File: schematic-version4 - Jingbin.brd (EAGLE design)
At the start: 47 x 28 mm, 54 parts, among them J2 FTDI_DEVICE, M1 WIRELESS-NRF24L01, Q1 8MHz, T1 NMOS, T2 NMOS, T3 NMOS, T4 NMOS, U1 ATMEGA328P_TQFP, U2 GY-521MPU6050

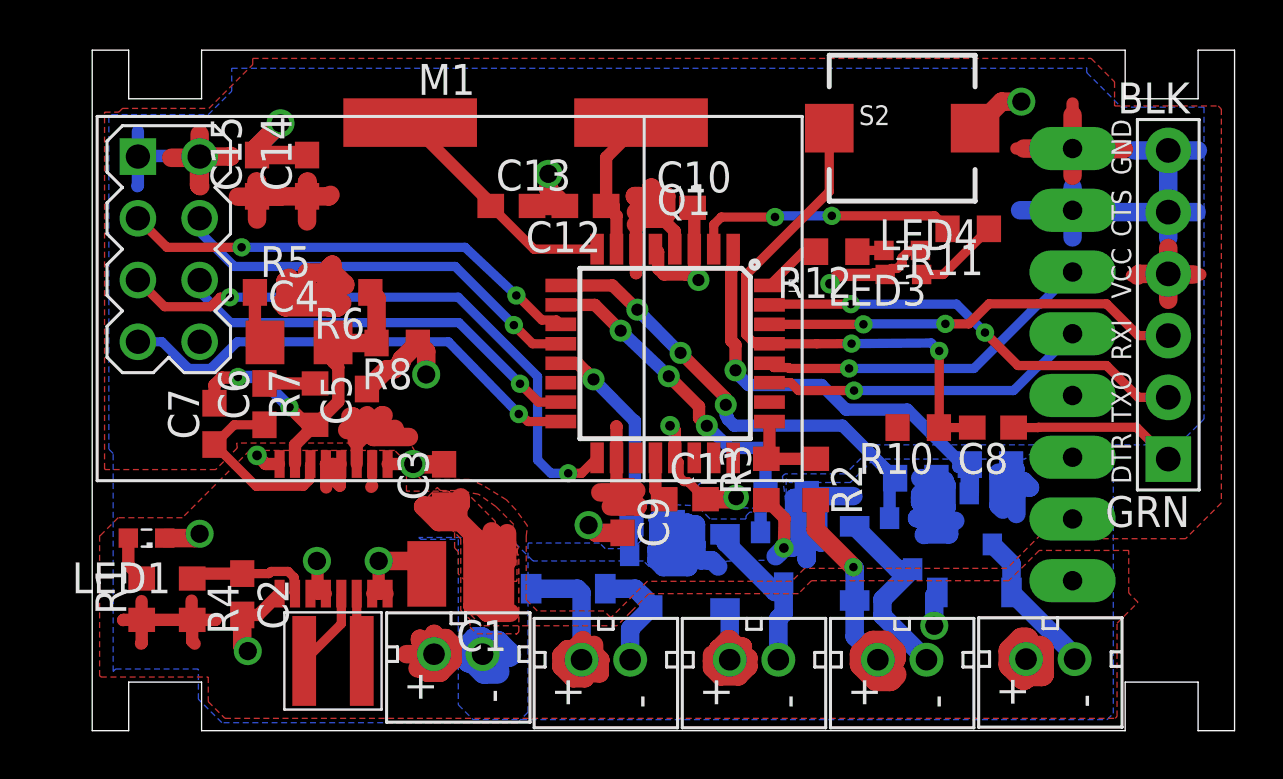
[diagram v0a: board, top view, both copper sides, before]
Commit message: Version 4 complete
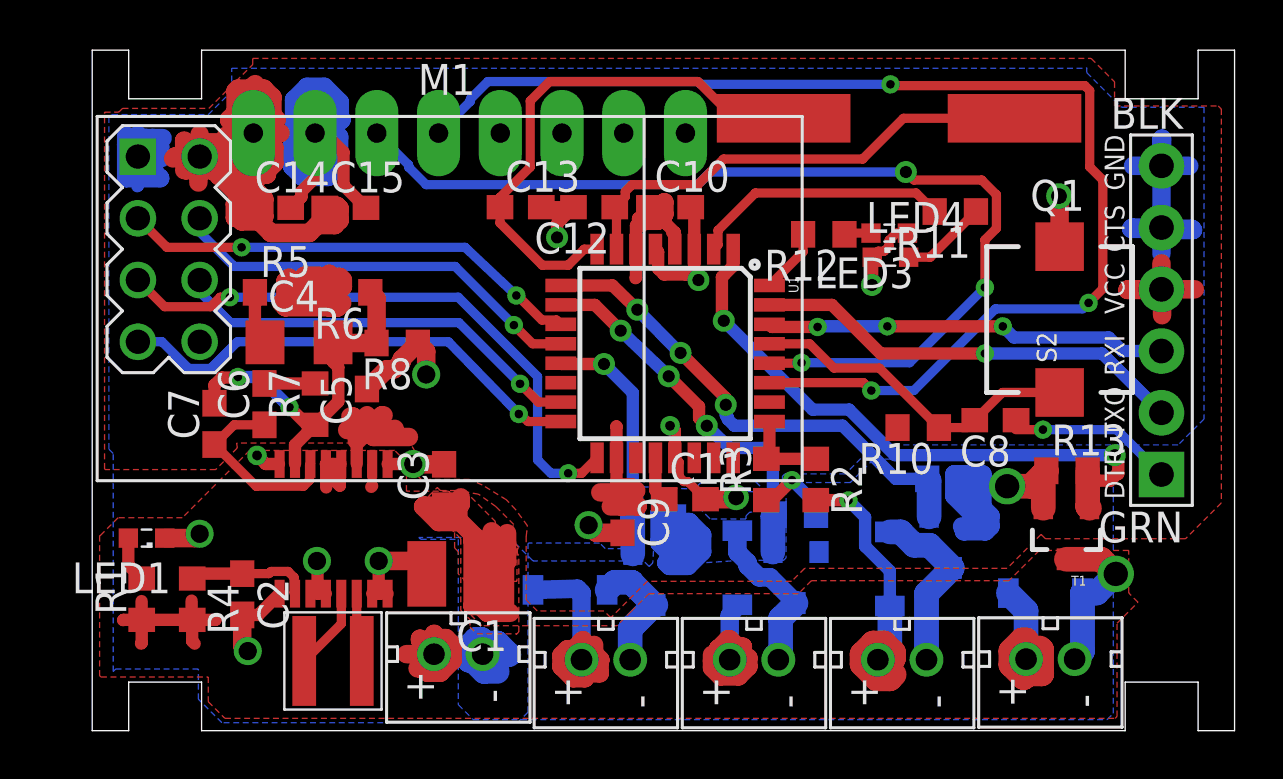
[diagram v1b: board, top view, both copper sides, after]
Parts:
- moved U2 15.9 mm to (15.5, 15.7), turned to 270 degrees
- moved Q1 15.4 mm to (33.2, 25.2)
- moved S2 10.2 mm to (39.8, 16.9), turned to 90 degrees
- moved C15 3.86 mm to (10.4, 21.5), turned to 0 degrees
- moved R13 3.16 mm to (40.1, 10.7), flipped to the top
- moved T1 3.11 mm to (40.1, 8.15), flipped to the top
- moved D1 2.92 mm to (39.2, 5.66)
- moved C14 2.02 mm to (7.32, 21.5), turned to 0 degrees
- moved T2 1.63 mm to (35.4, 7.80)
- moved D2 1.47 mm to (32.8, 6.68)
- moved R14 1.32 mm to (35.2, 10.4)
- moved T3 0.96 mm to (29.0, 6.35)
- moved R15 0.92 mm to (28.9, 8.89)
- moved LED3 0.89 mm to (32.8, 20.5)
- moved R12 0.89 mm to (30.1, 20.4)
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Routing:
- net SDA: track 13.6 -> 51.8 mm, vias 1 -> 3
- net V_REG_OUT: track 59.7 -> 86.8 mm
- net SCL: track 14.2 -> 41.2 mm, vias 1 -> 3
- net N$1: track 6.15 -> 19.8 mm
- net N$4: track 9.91 -> 21.9 mm
- net N$2: track 22.7 -> 14.0 mm, vias 2 -> 0
- net GND: track 113.2 -> 121.2 mm
- net PWM1: track 17.8 -> 25.5 mm, vias 1 -> 2
- net PWR: track 74.2 -> 77.1 mm, vias 2 -> 1
- net DTR: track 6.91 -> 8.03 mm, vias 0 -> 1
- net PWM3: track 14.6 -> 15.6 mm
- net N$5: track 8.11 -> 7.39 mm
- net N$3: track 6.12 -> 6.83 mm, vias 0 -> 1
- net RXD: track 17.3 -> 16.6 mm, vias 2 -> 3
- net PWM2: track 19.7 -> 20.4 mm
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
